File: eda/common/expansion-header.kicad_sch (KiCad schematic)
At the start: 10 parts, among them J2 Bus expansion

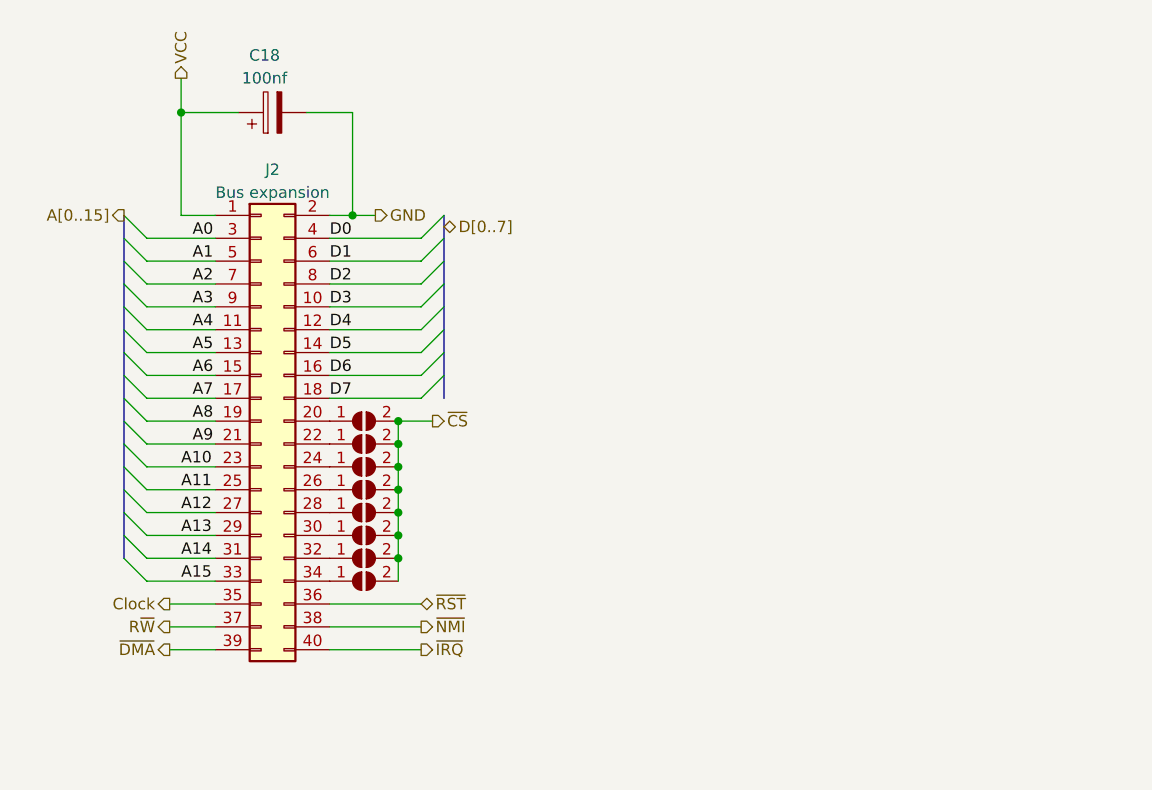
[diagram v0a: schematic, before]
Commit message: Sync
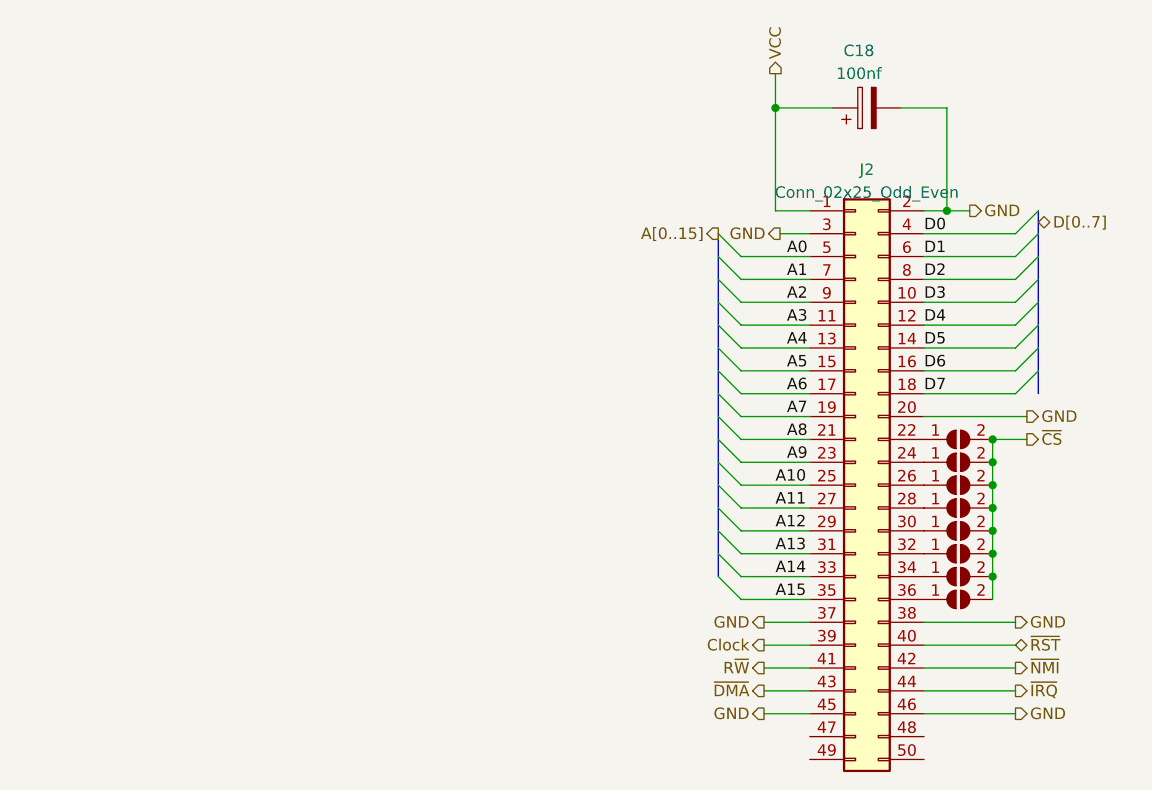
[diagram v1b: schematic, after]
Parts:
- removed J2: Bus expansion, Connector_PinHeader_2.54mm:PinHeader_2x20_P2.54mm_Horizontal, symbol Connector_Generic:Conn_02x20_Odd_Even
- added J2: Conn_02x25_Odd_Even, Connector_PinHeader_2.54mm:PinHeader_2x25_P2.54mm_Horizontal, symbol Connector_Generic:Conn_02x25_Odd_Even
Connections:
- net A0: now also J2.5 (Pin_5)
- net A1: now also J2.7 (Pin_7)
- net A10: now also J2.25 (Pin_25)
- net A11: now also J2.27 (Pin_27)
- net A12: now also J2.29 (Pin_29)
- net A13: now also J2.31 (Pin_31)
- net A14: now also J2.33 (Pin_33)
- net A15: now also J2.35 (Pin_35)
- net A2: now also J2.9 (Pin_9)
- net A3: now also J2.11 (Pin_11)
- net A4: now also J2.13 (Pin_13)
- net A5: now also J2.15 (Pin_15)
- net A6: now also J2.17 (Pin_17)
- net A7: now also J2.19 (Pin_19)
- net A8: now also J2.21 (Pin_21)
- net A9: now also J2.23 (Pin_23)
- net Clock: now also J2.39 (Pin_39)
- net D0: now also J2.4 (Pin_4)
- net D1: now also J2.6 (Pin_6)
- net D2: now also J2.8 (Pin_8)
- net D3: now also J2.10 (Pin_10)
- net D4: now also J2.12 (Pin_12)
- net D5: now also J2.14 (Pin_14)
- net D6: now also J2.16 (Pin_16)
- net D7: now also J2.18 (Pin_18)
- net GND: now also J2.2 (Pin_2), J2.20 (Pin_20), J2.3 (Pin_3), J2.37 (Pin_37), J2.38 (Pin_38), J2.45 (Pin_45), J2.46 (Pin_46)
- net R~{W}: now also J2.41 (Pin_41)
- net VCC: now also J2.1 (Pin_1)
- net ~{DMA}: now also J2.43 (Pin_43)
- net ~{IRQ}: now also J2.44 (Pin_44)
- net ~{NMI}: now also J2.42 (Pin_42)
- net ~{RST}: now also J2.40 (Pin_40)
- net at JP1.1 (A): now also J2.22 (Pin_22)
- net at JP2.1 (A): now also J2.24 (Pin_24)
- net at JP3.1 (A): now also J2.26 (Pin_26)
- net at JP4.1 (A): now also J2.28 (Pin_28)
- net at JP5.1 (A): now also J2.30 (Pin_30)
- net at JP6.1 (A): now also J2.32 (Pin_32)
- net at JP7.1 (A): now also J2.34 (Pin_34)
- net at JP8.1 (A): now also J2.36 (Pin_36)
